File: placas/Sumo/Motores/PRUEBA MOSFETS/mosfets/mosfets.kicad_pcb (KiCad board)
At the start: 2 copper layers, 54.6 x 45 mm, 17 parts, among them J1 Screw_Terminal_01x02, J3 Screw_Terminal_01x02, J5 Conn_01x06_Pin, Q1 IRLZ44N, Q2 IRLZ44N, Q3 IRLZ44N, Q4 IRLZ44N, U1 HIP4082xP

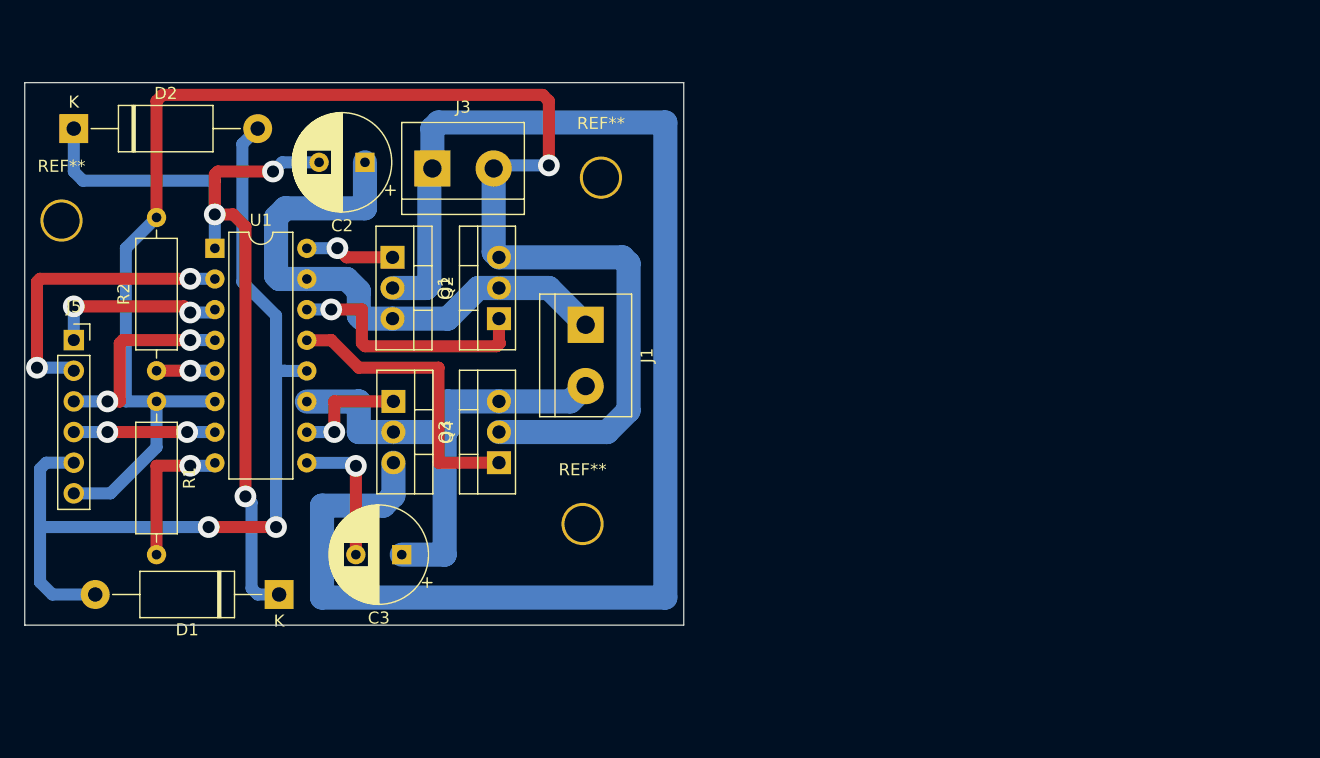
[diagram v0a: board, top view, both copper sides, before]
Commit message: dfg
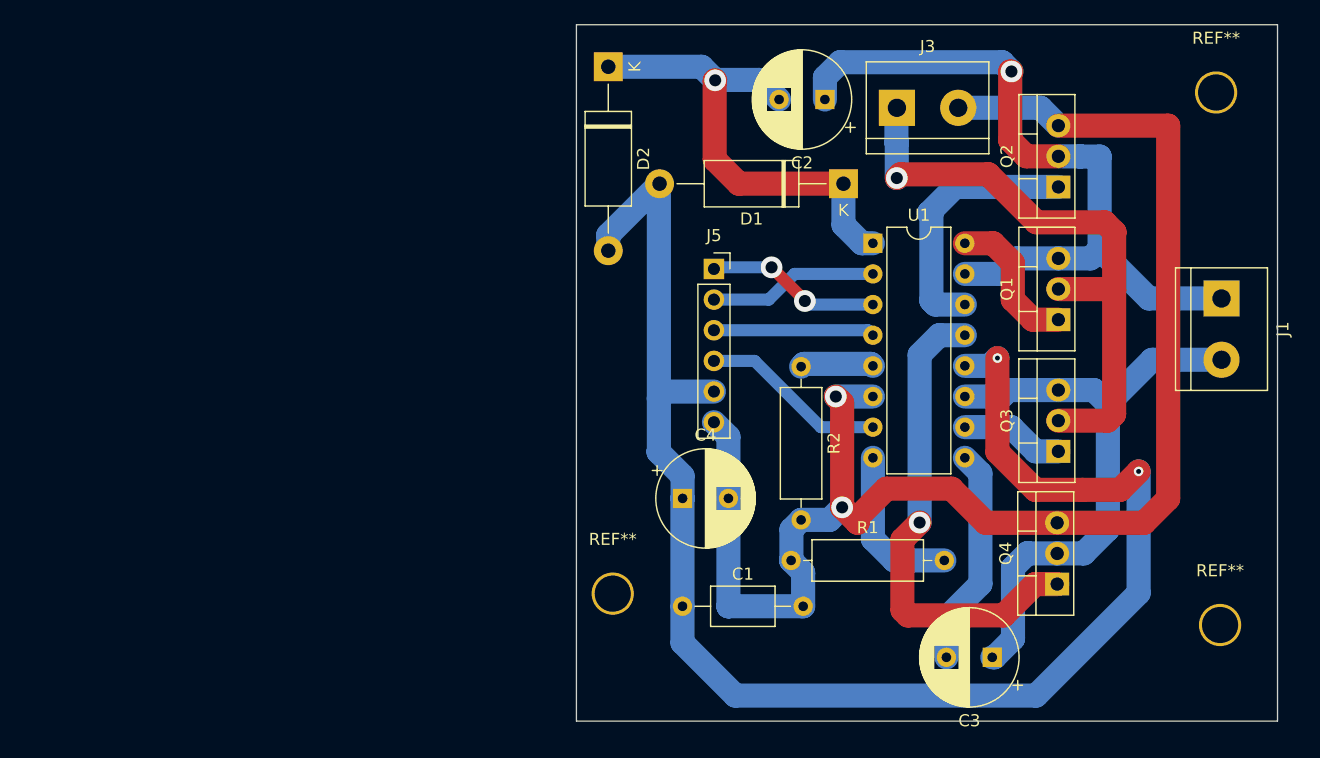
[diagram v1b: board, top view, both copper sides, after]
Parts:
- added C1: C, Capacitor_THT:C_Axial_L5.1mm_D3.1mm_P10.00mm_Horizontal, F.Cu at (113.7, 58.9)
- added C4: 47nf, Capacitor_THT:CP_Radial_D8.0mm_P3.80mm, F.Cu at (113.7, 50.0)
- C2, C3: value C_Polarized -> 47nf
- R1, R2: value R -> 36k
- moved REF** 101.7 mm to (158.2, 60.4)
- moved D1 57.8 mm to (127.0, 23.9)
- moved Q1 55.4 mm to (144.8, 35.1), turned to 90 degrees
- moved Q3 55.3 mm to (144.8, 46.0), turned to 90 degrees
- moved U1 54.5 mm to (129.5, 28.8)
- moved R1 54.2 mm to (122.7, 55.1), turned to 0 degrees
- moved R2 53.4 mm to (123.5, 39.0), turned to -90 degrees
- moved J5 53.4 mm to (116.3, 30.9)
- moved J1 52.7 mm to (158.4, 33.4)
- moved REF** 51.5 mm to (157.9, 16.3)
- moved C3 49.7 mm to (139.4, 63.1)
- moved Q2 47.6 mm to (144.8, 24.1)
- moved Q4 47.3 mm to (144.7, 57.0)
- moved D2 44.6 mm to (107.5, 14.2), turned to -90 degrees
- moved J3 38.8 mm to (131.5, 17.6)
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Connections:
- Q3 pad 2: Net-(J1-Pin_2) -> VDD
- Q3 pad 3: VDD -> Net-(J1-Pin_2)
- Q4 pad 2: GND -> Net-(J1-Pin_2)
- Q4 pad 3: Net-(J1-Pin_2) -> GND
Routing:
- net VDD: track 120.1 -> 50.6 mm, vias 0 -> 1
- net +5V: track 74.2 -> 128.6 mm
- net Net-(D1-K): track 69.2 -> 39.9 mm, vias 3 -> 1
- net Net-(J1-Pin_1): track 46.9 -> 63.4 mm, vias 0 -> 1
- net Net-(Q4-G): track 24.7 -> 40.2 mm, vias 0 -> 1
- net Net-(J5-Pin_2): track 25.1 -> 14.1 mm, vias 2 -> 0
- net Net-(J1-Pin_2): track 42.3 -> 51.3 mm
- net Net-(U1-AHB): track 11.5 -> 18.2 mm, vias 1 -> 0
- net Net-(Q1-G): track 7.42 -> 12.2 mm, vias 1 -> 0
- net GND: track 130.7 -> 126.1 mm, vias 1 -> 2
- net Net-(J5-Pin_4): track 11.7 -> 15.4 mm, vias 2 -> 0
- net Net-(J5-Pin_3): track 16.6 -> 13.3 mm, vias 2 -> 0
- net Net-(U1-DEL): track 4.84 -> 6.11 mm, vias 1 -> 0
- net Net-(Q3-G): track 9.72 -> 8.58 mm, vias 1 -> 0
- net Net-(U1-DIS): track 12.3 -> 13.4 mm, vias 1 -> 0
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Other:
- board size 54.6 x 45 mm -> 58.1 x 57.7 mm
